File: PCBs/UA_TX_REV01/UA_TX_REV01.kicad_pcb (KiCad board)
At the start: 2 copper layers, 63.5 x 38.1 mm, 13 parts, among them J1 Screw_Terminal_01x03, J2 Screw_Terminal_01x02, U1 SeeeduinoXIAO, U3 AMS1117

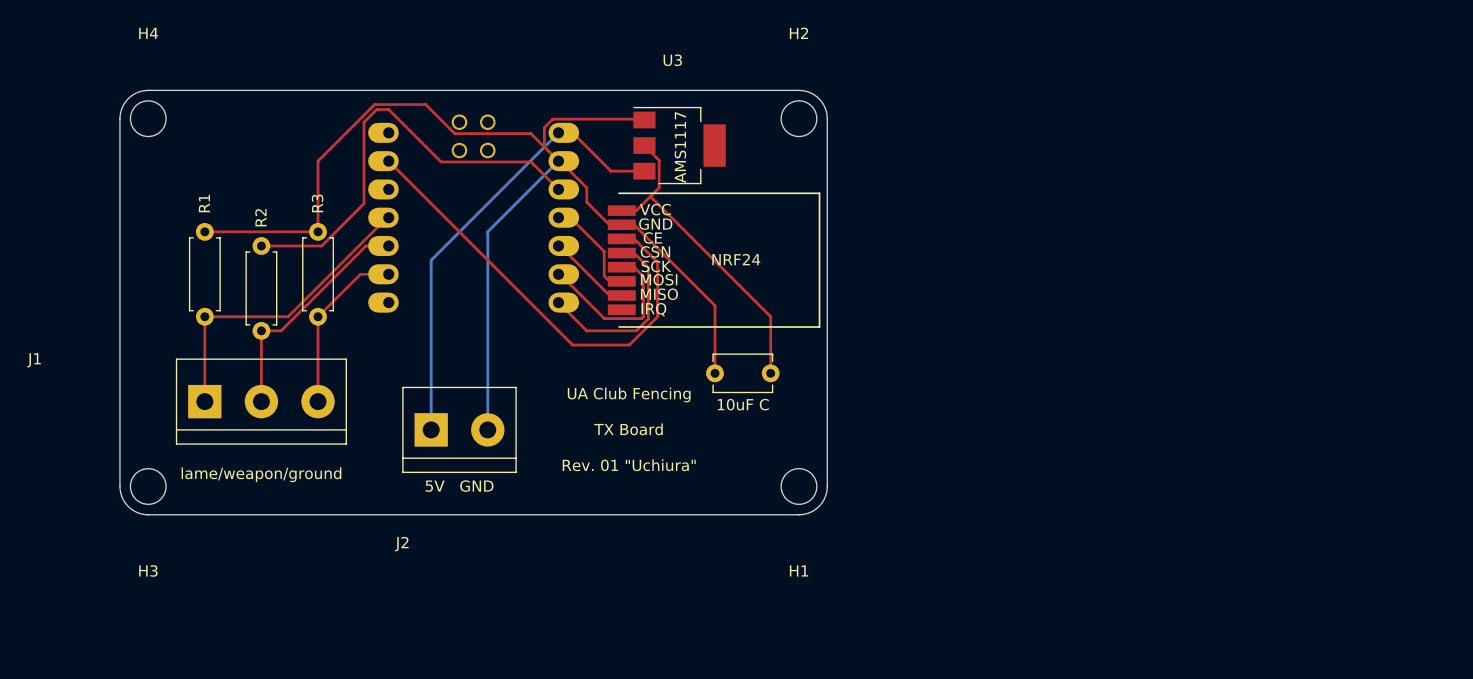
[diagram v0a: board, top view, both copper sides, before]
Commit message: stopped updates
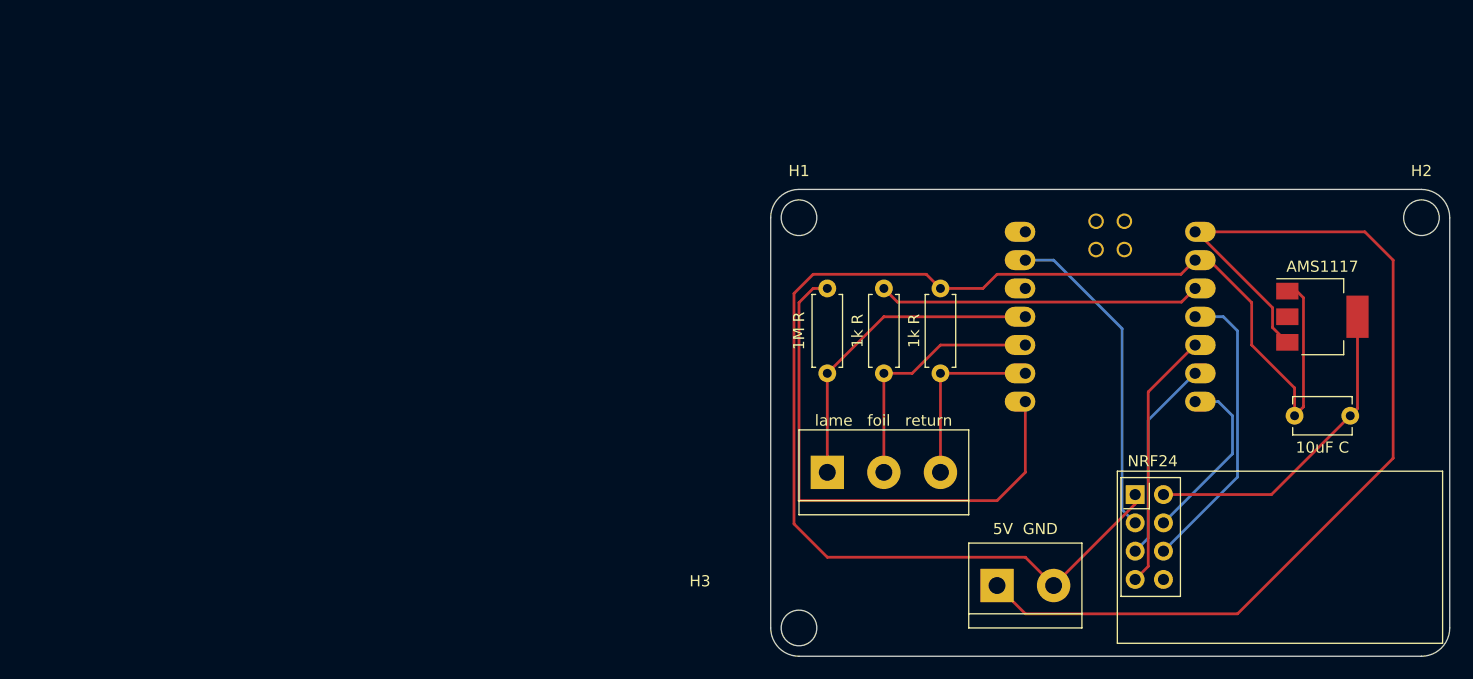
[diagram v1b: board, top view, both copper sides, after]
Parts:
- removed H4: MountingHole, MountingHole:MountingHole_3.2mm_M3
- removed J1: Screw_Terminal_01x03, TerminalBlock:TerminalBlock_bornier-3_P5.08mm
- removed J2: Screw_Terminal_01x02, TerminalBlock:TerminalBlock_bornier-2_P5.08mm
- removed R1, R2, R3: R, Resistor_THT:R_Axial_DIN0207_L6.3mm_D2.5mm_P7.62mm_Horizontal
- removed U3: AMS1117, Package_TO_SOT_SMD:SOT-223-3_TabPin2
- added 1M R: R, Resistor_THT:R_Axial_DIN0207_L6.3mm_D2.5mm_P7.62mm_Horizontal, F.Cu at (149.9, 86.4)
- added 1k R: R, Resistor_THT:R_Axial_DIN0207_L6.3mm_D2.5mm_P7.62mm_Horizontal, F.Cu at (160.0, 94.0)
- added 1k R: R, Resistor_THT:R_Axial_DIN0207_L6.3mm_D2.5mm_P7.62mm_Horizontal, F.Cu at (154.9, 94.0)
- added 5V  GND: Screw_Terminal_01x02, TerminalBlock:TerminalBlock_bornier-2_P5.08mm, F.Cu at (165.1, 113.0)
- added AMS1117: AMS1117-3.3, Package_TO_SOT_SMD:SOT-223-3_TabPin2, F.Cu at (194.3, 88.9)
- added lame   foil   return: Screw_Terminal_01x03, TerminalBlock:TerminalBlock_bornier-3_P5.08mm, F.Cu at (149.9, 102.9)
- NRF24: value nRF24L01_module -> NRF24L01_Breakout; footprint nrf24smd:NRF24L01-Module-SMD -> RF_Module:nRF24L01_Breakout
- moved H3 59.8 mm to (147.3, 116.8)
- moved U1 57.8 mm to (175.3, 88.9)
- moved H2 56.6 mm to (203.2, 80.0)
- moved 10uF C 52.2 mm to (196.8, 97.8)
- moved NRF24 50.0 mm to (177.5, 104.9), turned to 0 degrees
- moved H1 24.1 mm to (147.3, 80.0)
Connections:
- NRF24 pad 1: Net-(C1-Pad1) -> Net-(C1-Pad2)
- NRF24 pad 2: Net-(C1-Pad2) -> Net-(C1-Pad1)
- U1 pad 7: unconnected-(U1-Pad7) -> Net-(R1-Pad1)
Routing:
- net Net-(J2-Pad1): track 39.3 -> 92.4 mm
- net Net-(R1-Pad1): track 0.00 -> 48.6 mm
- net Net-(C1-Pad2): track 108.2 -> 126.3 mm
- net Net-(U1-Pad11): track 9.79 -> 26.9 mm
- net Net-(U1-Pad10): track 7.97 -> 23.3 mm
- net Net-(U2-Pad3): track 40.5 -> 29.2 mm
- net Net-(R2-Pad2): track 39.0 -> 29.0 mm
- net Net-(U1-Pad9): track 14.8 -> 18.2 mm
- net Net-(J1-Pad2): track 20.9 -> 22.6 mm
- net Net-(J1-Pad1): track 27.8 -> 28.8 mm
- net Net-(J1-Pad3): track 15.5 -> 16.5 mm
- net Net-(U1-Pad8): track 16.7 -> 16.1 mm
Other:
- board size 63.5 x 38.1 mm -> 61 x 41.9 mm
- board text removed: "5V GND"
- board text removed: "UA Club Fencing TX Board Rev. 01 {dblquote}Uchiura{dblquote}"
- board text removed: "lame/weapon/ground"
